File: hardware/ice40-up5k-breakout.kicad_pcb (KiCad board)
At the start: 2 copper layers, 20.3 x 68.6 mm, 37 parts, among them IC1 AT25SF321B-SSHB-T, J1 Conn_01x26, J3 Conn_01x26, SW1 220AMA04R, SW2 220AMA04R, SW4 220AMA04R, U1 AP2112K-3.3TRG1, U19 AP2112K-1.2TRG1, U2 AP2112K-2.5TRG1, U20 ICE40UP5K-SG48I

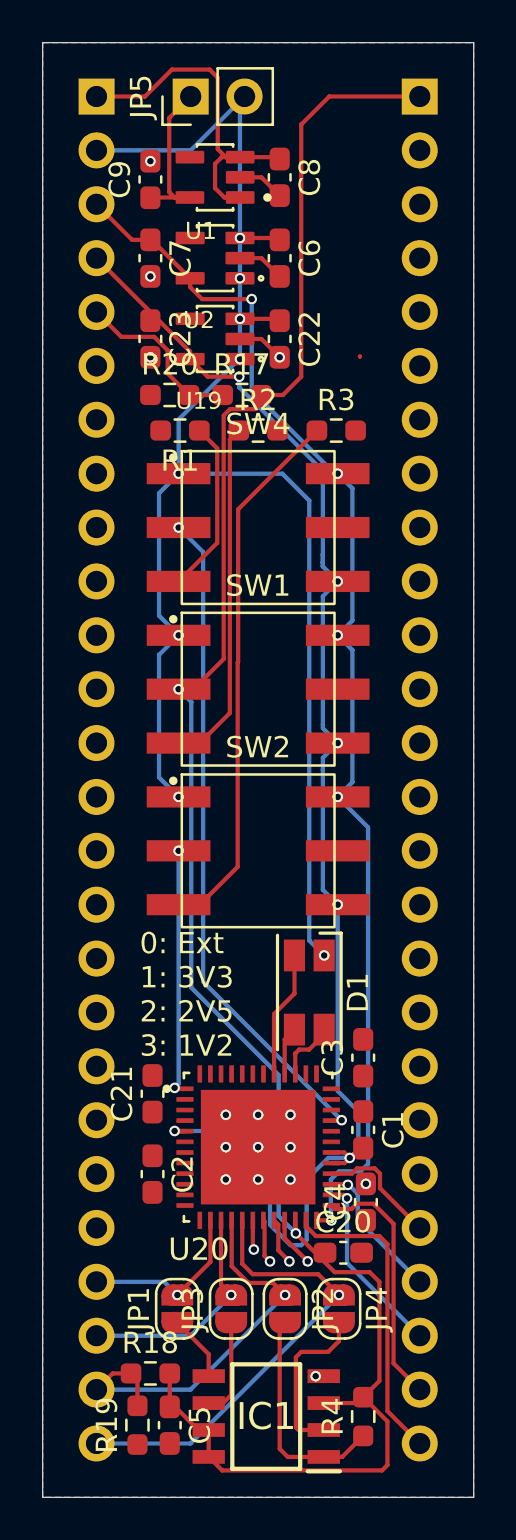
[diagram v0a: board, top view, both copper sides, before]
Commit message: Finalizes draft 1.
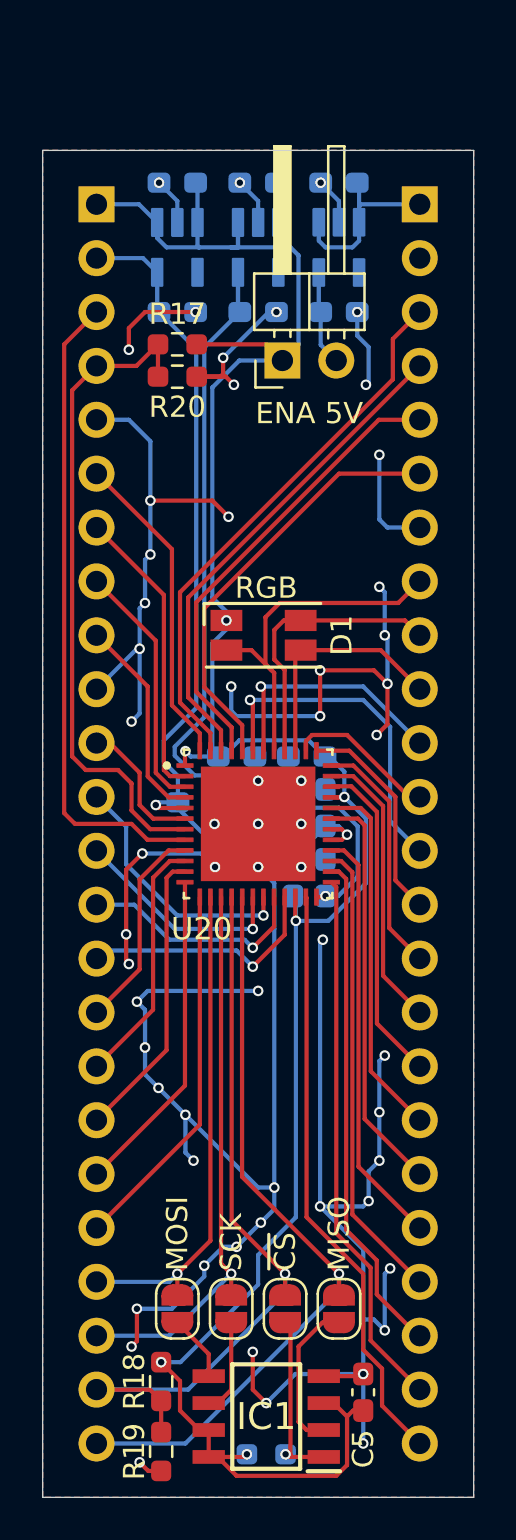
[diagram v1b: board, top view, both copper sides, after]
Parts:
- removed J3: Conn_01x26, Connector_PinHeader_2.54mm:PinHeader_1x26_P2.54mm_Vertical
- removed JP5: Jumper_2_Bridged, Connector_PinHeader_2.54mm:PinHeader_1x02_P2.54mm_Vertical
- removed R1, R2, R3: 100K, Resistor_SMD:R_0603_1608Metric_Pad0.98x0.95mm_HandSolder
- removed SW1, SW2, SW4: 220AMA04R, compi:220AMA04R
- added 5V_ENA1: Jumper_2_Bridged, Connector_PinHeader_2.54mm:PinHeader_1x02_P2.54mm_Horizontal, F.Cu at (123.1, 65.8)
- added J2: Conn_01x24, Connector_PinHeader_2.54mm:PinHeader_1x24_P2.54mm_Vertical, B.Cu at (129.5, 58.4)
- C1, C2, C20, C21, C22, C23, C3, C4, C6, C7, C8, C9, R4, U1, U19, U2: moved to B.Cu
- J1: value Conn_01x26 -> Conn_01x24; footprint Connector_PinHeader_2.54mm:PinHeader_1x26_P2.54mm_Vertical -> Connector_PinHeader_2.54mm:PinHeader_1x24_P2.54mm_Vertical
- moved C2 19.1 mm to (125.1, 86.9), turned to 90 degrees
- moved C20 17.8 mm to (123.6, 90.2), turned to 90 degrees
- moved C1 17.3 mm to (119.0, 86.6), turned to 0 degrees
- moved D1 17.0 mm to (122.2, 78.7), turned to 0 degrees
- moved C21 16.4 mm to (120.9, 84.5), turned to 0 degrees
- moved C4 15.4 mm to (125.1, 90.2)
- moved U20 15.2 mm to (121.9, 87.6)
- moved C3 14.4 mm to (124.2, 84.5), turned to 180 degrees
- moved C9 10.9 mm to (125.7, 63.5), turned to 0 degrees
- moved C5 9.25 mm to (126.9, 114.4), turned to 90 degrees
- moved C22 8.81 mm to (118.1, 57.4), turned to 180 degrees
- moved U1 6.71 mm to (125.7, 60.5), turned to -90 degrees
- moved C7 5.68 mm to (121.9, 63.5), turned to 0 degrees
- moved J1 5.08 mm to (114.3, 58.4)
- moved R4 4.91 mm to (122.3, 117.3), turned to 180 degrees
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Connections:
- C20 pad 1: VCC_BANK1 -> +3V3
- C21 pad 1: VCC_BANK2 -> +3V3
- C3 pad 1: VCC_BANK0 -> +3V3
- C5 pad 1: VCC_BANK1 -> +3V3
- D1 pad 3: /IO_B0_RGB1 -> /IO_B0_RGB0
- D1 pad 4: /IO_B0_RGB0 -> /IO_B0_RGB1
- IC1 pad 3: VCC_BANK1 -> +3V3
- IC1 pad 7: VCC_BANK1 -> +3V3
- IC1 pad 8: VCC_BANK1 -> +3V3
- J1 pad 1: +5V -> +3V3
- J1 pad 10: /IO_B2_3 -> GND
- J1 pad 11: /IO_B2_4 -> /IO_B1_13
- J1 pad 12: GND -> /IO_B1_29
- J1 pad 14: /IO_B1_29 -> /IO_B1_25
- J1 pad 15: /IO_B1_25 -> /IO_B1_23
- J1 pad 16: /IO_B1_24 -> /IO_B1_16
- J1 pad 17: /IO_B1_23 -> /IO_B1_18
- J1 pad 18: /IO_B1_22 -> /IO_B1_20
- J1 pad 19: /IO_B1_20 -> /IO_B1_22
- J1 pad 2: +3V3 -> +1V2
- J1 pad 20: /IO_B1_18 -> /IO_B1_24
- J1 pad 21: /IO_B1_16 -> /IO_B1_SPI_SO
- J1 pad 22: /IO_B1_13 -> /IO_B1_SPI_SCK
- J1 pad 23: /IO_B1_SPI_SO -> /IO_B1_SPI_~{CS}
- J1 pad 24: /IO_B1_SPI_SCK -> /IO_B1_SPI_SI
- J1 pad 3: +2V5 -> /CDONE
- J1 pad 4: +1V2 -> /~{CRES}
- J1 pad 5: /~{CRES} -> GND
- J1 pad 6: /CDONE -> /IO_B2_4
- J1 pad 7: GND -> /IO_B2_6
- J1 pad 8: /IO_B2_0 -> /IO_B2_9
- J1 pad 9: /IO_B2_2 -> /IO_B2_8
- R17 pad 2: VCC_BANK1 -> +3V3
- R18 pad 2: VCC_BANK1 -> +3V3
- R4 pad 2: VCC_BANK1 -> +3V3
- U20 pad 1: VCC_BANK2 -> +3V3
- U20 pad 22: VCC_BANK1 -> +3V3
- U20 pad 33: VCC_BANK0 -> +3V3
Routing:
- net GND: track 7.06 -> 175.7 mm, vias 15 -> 60
- net VCC_BANK1: track 95.7 -> 0.00 mm, vias 2 -> 0
- net +3V3: track 76.1 -> 112.6 mm, vias 8 -> 6
- net VCC_BANK0: track 31.6 -> 0.00 mm, vias 2 -> 0
- net /CDONE: track 0.00 -> 30.5 mm
- net +1V2: track 69.1 -> 42.8 mm, vias 6 -> 2
- net /IO_B2_2: track 0.00 -> 26.0 mm
- net Net-(R3-Pad1): track 25.6 -> 0.00 mm
- net /IO_B2_0: track 0.00 -> 23.3 mm
- net /~{CRES}: track 8.21 -> 31.2 mm
- net /IO_B2_5: track 0.00 -> 21.8 mm
- net /IO_B2_3: track 0.00 -> 20.2 mm
- net +2V5: track 58.4 -> 38.7 mm, vias 5 -> 1
- net /IO_B0_42: track 0.00 -> 19.2 mm
- net /IO_B1_24: track 0.00 -> 17.6 mm
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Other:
- board size 20.3 x 68.6 mm -> 20.3 x 63.5 mm
- board text added: "ENA 5V"
- board text added: "MISO"
- board text added: "MOSI"
- board text added: "RGB"
- board text added: "SCK"
- board text added: "~{CS}"
- board text removed: "0: Ext 1: 3V3 2: 2V5 3: 1V2"
